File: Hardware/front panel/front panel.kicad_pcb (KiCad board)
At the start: 2 copper layers, 103 x 49.6 mm, 0 parts

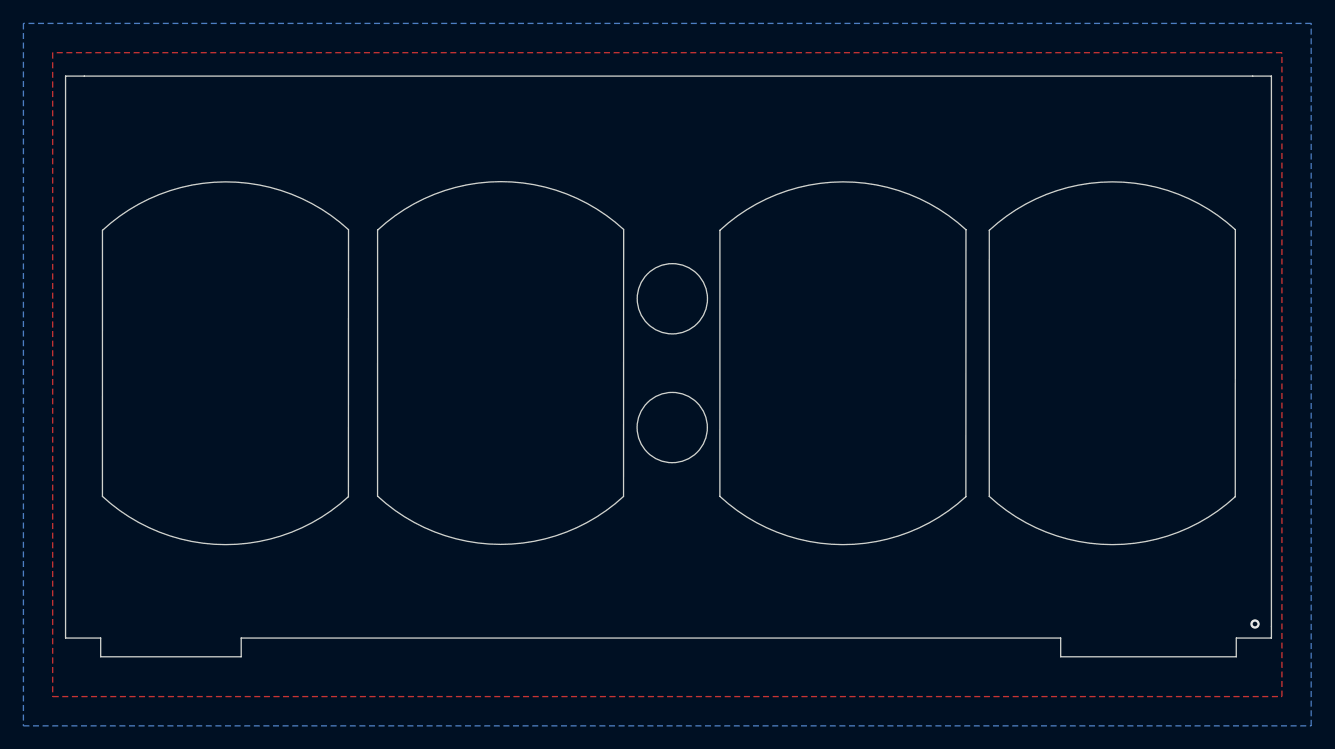
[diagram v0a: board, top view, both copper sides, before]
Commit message: Major HW and FW improvements
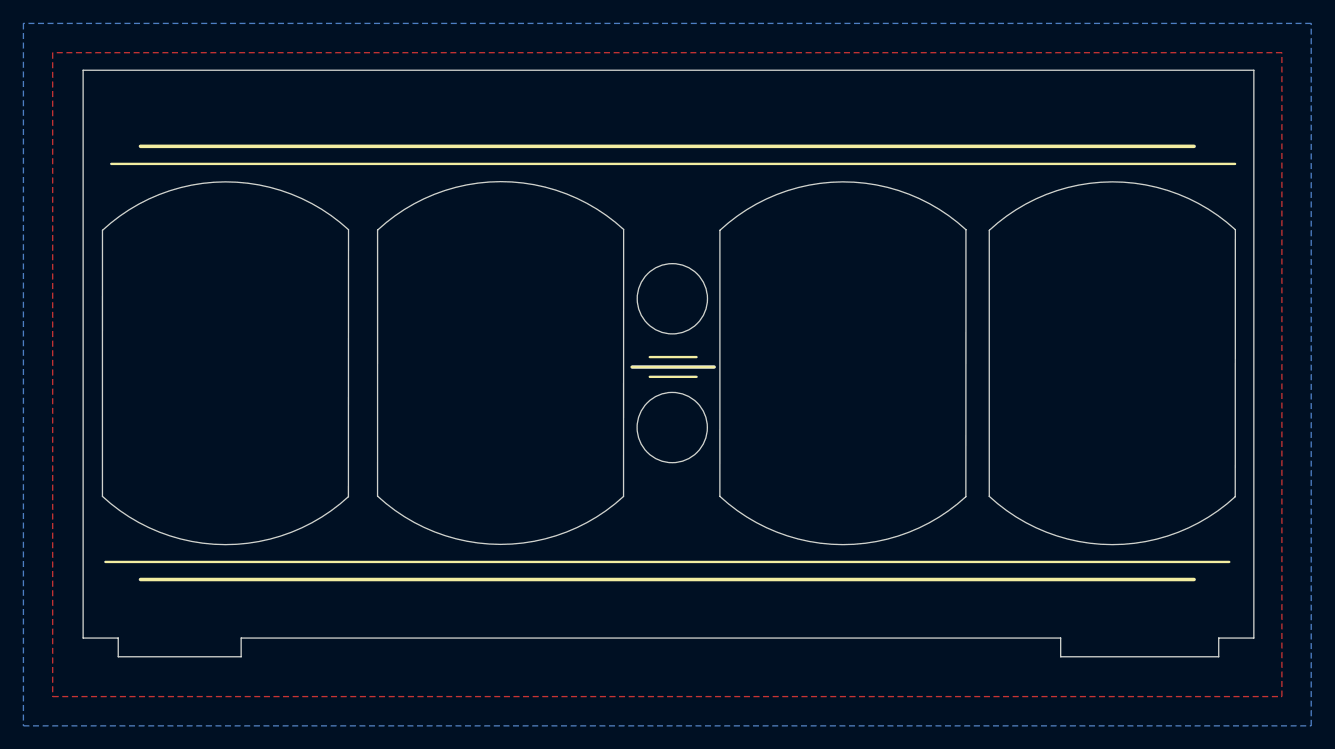
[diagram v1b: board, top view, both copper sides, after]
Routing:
- net (no net): vias 1 -> 0
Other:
- board size 103 x 49.6 mm -> 100 x 50.1 mm
- rule pad_to_mask_clearance: 0.051 -> 0
